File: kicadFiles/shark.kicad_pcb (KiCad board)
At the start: 2 copper layers, 225.6 x 74.8 mm, 259 parts, among them J1 USB_C_Receptacle, Q1 AO4406AL, SW1 MXSwitch, SW10 MXSwitch, SW11 MXSwitch, SW12 MXSwitch, SW13 MXSwitch, SW14 MXSwitch, SW15 MXSwitch, SW16 MXSwitch, SW17 MXSwitch, SW18 MXSwitch, SW19 MXSwitch, SW2 MXSwitch, SW20 MXSwitch, SW21 MXSwitch, SW22 MXSwitch, SW23 MXSwitch, SW24 MXSwitch, SW25 MXSwitch, SW26 MXSwitch, SW27 MXSwitch, SW28 MXSwitch, SW29 MXSwitch, SW3 MXSwitch, SW30 MXSwitch, SW31 MXSwitch, SW32 MXSwitch, SW33 MXSwitch, SW34 MXSwitch, SW35 MXSwitch, SW36 MXSwitch, SW37 MXSwitch, SW38 MXSwitch, SW39 MXSwitch, SW4 MXSwitch, SW40 MXSwitch, SW41 MXSwitch, SW42 MXSwitch, SW43 MXSwitch, SW44 MXSwitch, SW45 MXSwitch, SW46 MXSwitch, SW47 MXSwitch, SW48 MXSwitch, SW49 MXSwitch, SW5 MXSwitch, SW50 MXSwitch, SW51 MXSwitch, SW6 MXSwitch, SW7 MXSwitch, SW8 MXSwitch, SW9 MXSwitch, U1 STM32F303CCT7, U2 MCP1700-3302E_SOT23, Y1 8MHz

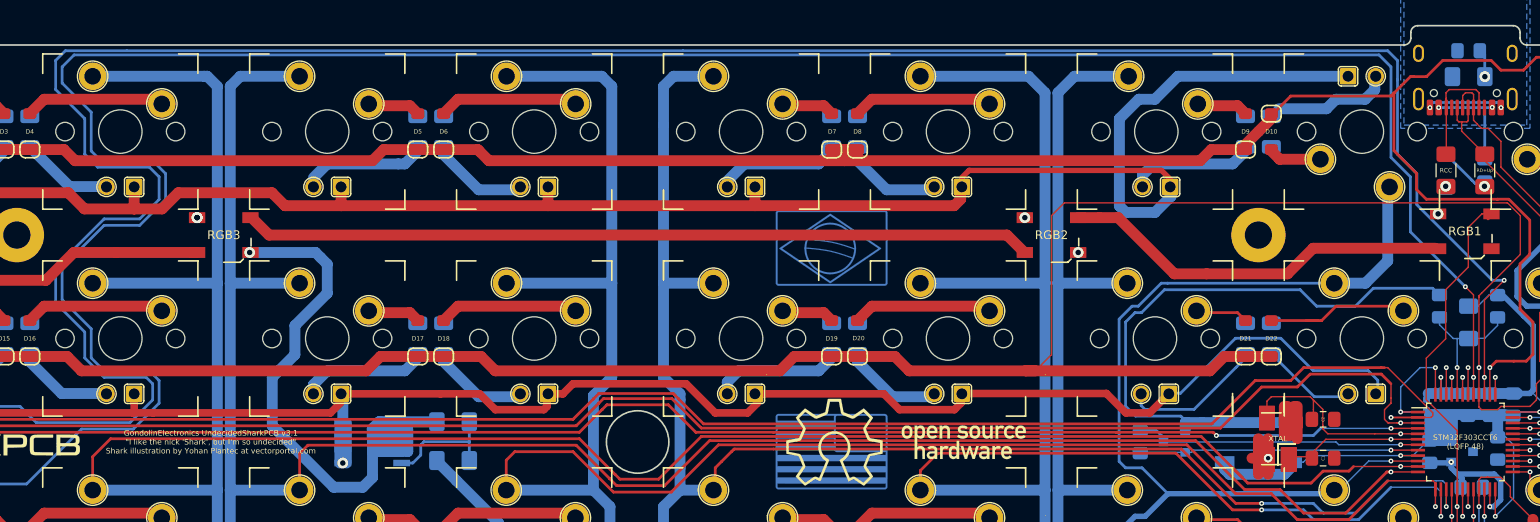
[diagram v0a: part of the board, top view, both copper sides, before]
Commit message: Reorganized folders
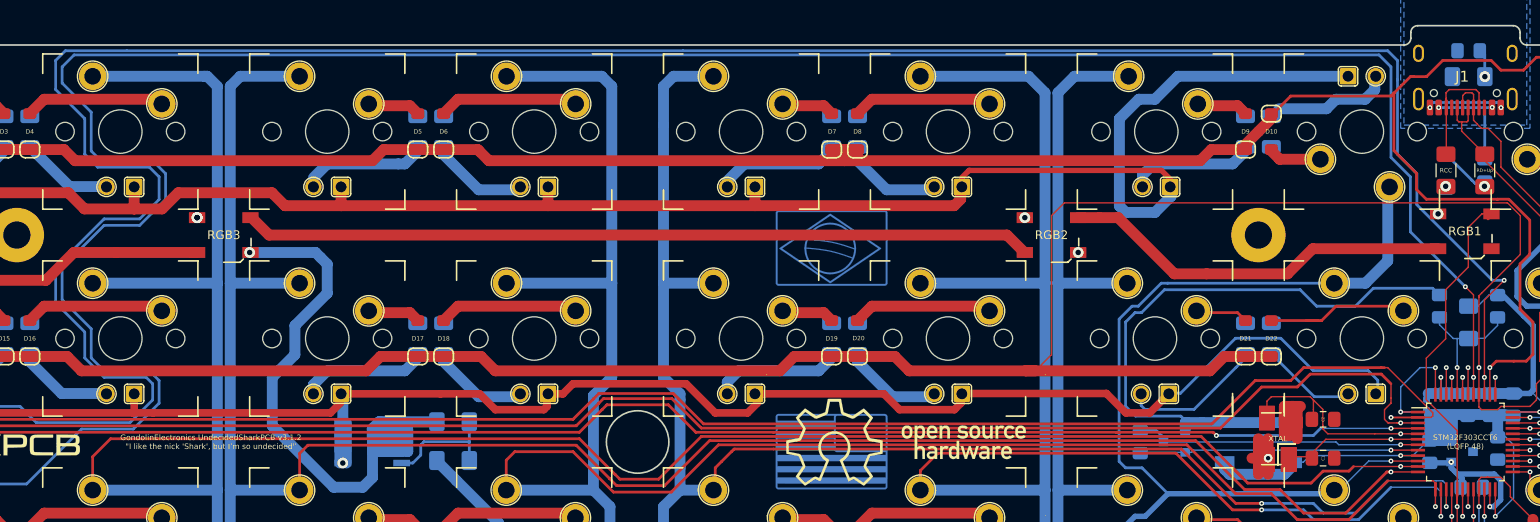
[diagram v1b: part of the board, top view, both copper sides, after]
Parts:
- removed the Y1 at (207.2, 102.4) (x2)
- added Y1 (x2): 8MHz, acheronComponents:Crystal_SMD_5032-4Pin_5.0x3.2mm, F.Cu at (207.2, 102.4)
- D1, D10, D11, D12, D13, D14, D15, D16, D17, D18, D19, D2, D20, D21, D22, D23, D24, D25, D26, D27, D28, D29, D3, D30, D31, D32, D33, D34, D35, D36, D37, D38, D39, D4, D40, D41, D42, D43, D44, D45, D46, D47, D48, D5, D6, D7, D8, D9: footprint Keyboard_switches:D_SOD-123 -> acheronComponents:D_SOD-123
- J1: footprint USBconnector:TYPE-C-31-M-13 -> acheronConnectors:TYPE-C-31-M-12
- ROT1: footprint encoders:ALPS_EC11E -> acheronHardware:ALPS_EC11E
- SW1, SW10, SW11, SW12, SW13, SW14, SW15, SW16, SW17, SW18, SW19, SW2, SW20, SW21, SW22, SW23, SW24, SW25, SW26, SW27, SW28, SW29, SW3, SW30, SW31, SW32, SW33, SW34, SW35, SW36, SW37, SW38, SW39, SW4, SW40, SW41, SW42, SW43, SW44, SW45, SW46, SW47, SW48, SW5, SW6, SW7, SW8, SW9: footprint Keyboard_switches:MX100 -> acheronKeyboardSwitches:MX100
- SW49, SW50, SW51: footprint Keyboard_switches:MX200R -> acheronKeyboardSwitches:MX200R
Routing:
- net GND: track 170.8 -> 172.5 mm
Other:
- board text added: "GondolinElectronics UndecidedSharkPCB v3.1.2 "I like the nick 'Shark', but I'm so undecided""
- board text removed: "GondolinElectronics UndecidedSharkPCB v3.1 "I like the nick 'Shark', but I'm so undecided" Shark illustration by Yohan Plantec at vectorportal.com"
